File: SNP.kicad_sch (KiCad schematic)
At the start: 9 parts, among them J1 SNP, U75 IN74ALS32N (КР1533ЛЛ1)

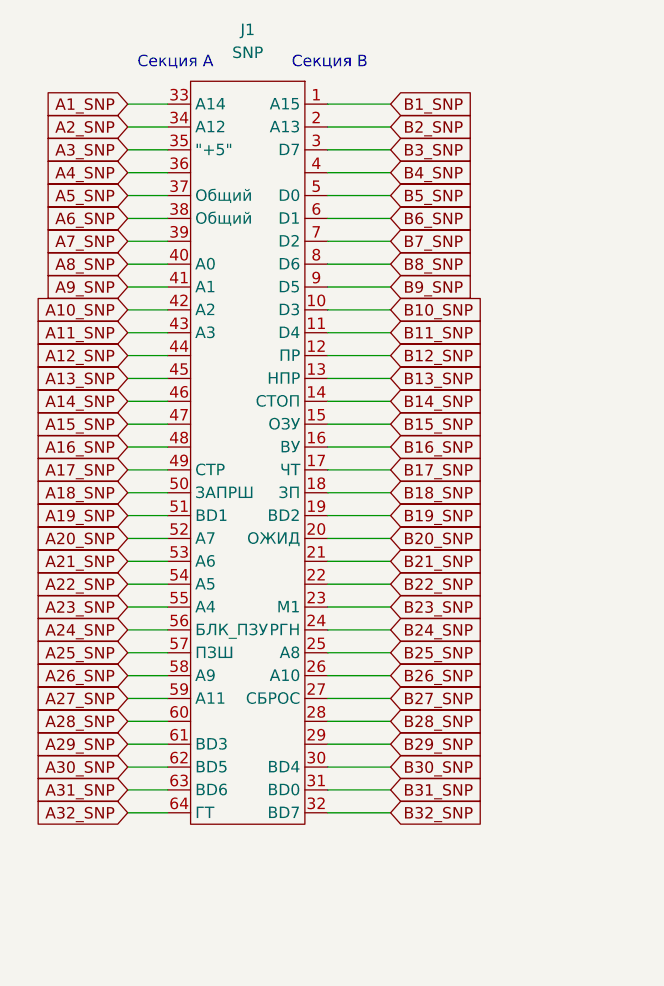
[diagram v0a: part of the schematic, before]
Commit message: March 22nd - 3rd edition
List 3 is complete
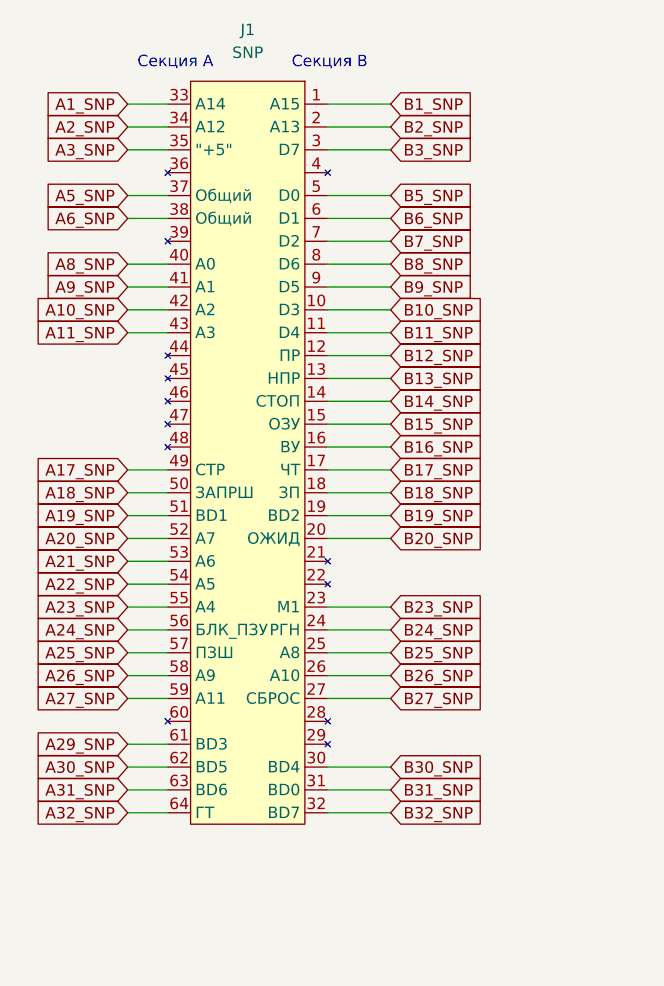
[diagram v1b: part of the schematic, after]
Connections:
- net GND: no longer J1.45
- net A12_SNP: no longer names the net of J1.44
- net A14_SNP: no longer names the net of J1.46
- net A15_SNP: no longer names the net of J1.47
- net A16_SNP: no longer names the net of J1.48
- net A28_SNP: no longer names the net of J1.60
- net A4_SNP: no longer names the net of J1.36
- net A7_SNP: no longer names the net of J1.39
- net B21_SNP: no longer names the net of J1.21
- net B22_SNP: no longer names the net of J1.22
- net B28_SNP: no longer names the net of J1.28
- net B29_SNP: no longer names the net of J1.29
- net B4_SNP: no longer names the net of J1.4
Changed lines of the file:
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@@
 (kicad_sch (version 20211123) (generator eeschema)
-  (paper "A3")
+  (paper "A4")
   (title_block
     (comment 2 "Евстафьев")
@@
     (stroke (width 0) (type default) (color 0 0 0 0))
   )
-  (wire (pts (xy 40.005 69.85) (xy 44.45 69.85))
-    (stroke (width 0) (type default) (color 0 0 0 0))
-  )
   (wire (pts (xy 173.99 46.355) (xy 173.99 50.165))
     (stroke (width 0) (type default) (color 0 0 0 0))
@@
     (stroke (width 0) (type default) (color 0 0 0 0))
   )
-  (wire (pts (xy 40.005 67.31) (xy 44.45 67.31))
-    (stroke (width 0) (type default) (color 0 0 0 0))
-  )
   (wire (pts (xy 138.43 46.355) (xy 138.43 70.485))
     (stroke (width 0) (type default) (color 0 0 0 0))
@@
     (stroke (width 0) (type default) (color 0 0 0 0))
   )
-  (wire (pts (xy 40.005 64.77) (xy 44.45 64.77))
-    (stroke (width 0) (type default) (color 0 0 0 0))
-  )
   (wire (pts (xy 128.27 46.355) (xy 128.27 60.325))
     (stroke (width 0) (type default) (color 0 0 0 0))
   )
-  (wire (pts (xy 69.215 85.09) (xy 62.23 85.09))
-    (stroke (width 0) (type default) (color 0 0 0 0))
-  )
   (wire (pts (xy 40.005 74.93) (xy 44.45 74.93))
     (stroke (width 0) (type default) (color 0 0 0 0))
@@
     (stroke (width 0) (type default) (color 0 0 0 0))
   )
-  (wire (pts (xy 69.215 102.87) (xy 62.23 102.87))
-    (stroke (width 0) (type default) (color 0 0 0 0))
-  )
   (wire (pts (xy 135.89 67.945) (xy 151.13 67.945))
     (stroke (width 0) (type default) (color 0 0 0 0))
@@
     (stroke (width 0) (type default) (color 0 0 0 0))
   )
-  (wire (pts (xy 40.005 62.23) (xy 44.45 62.23))
-    (stroke (width 0) (type default) (color 0 0 0 0))
-  )
   (wire (pts (xy 133.35 46.355) (xy 133.35 65.405))
     (stroke (width 0) (type default) (color 0 0 0 0))
@@
     (stroke (width 0) (type default) (color 0 0 0 0))
   )
-  (wire (pts (xy 40.005 49.53) (xy 44.45 49.53))
-    (stroke (width 0) (type default) (color 0 0 0 0))
-  )
   (wire (pts (xy 124.46 88.265) (xy 151.13 88.265))
     (stroke (width 0) (type default) (color 0 0 0 0))
@@
     (stroke (width 0) (type default) (color 0 0 0 0))
   )
-  (wire (pts (xy 69.215 105.41) (xy 62.23 105.41))
-    (stroke (width 0) (type default) (color 0 0 0 0))
-  )
   (wire (pts (xy 128.27 98.425) (xy 128.27 100.965))
     (stroke (width 0) (type default) (color 0 0 0 0))
@@
     (stroke (width 0) (type default) (color 0 0 0 0))
   )
-  (wire (pts (xy 40.005 72.39) (xy 44.45 72.39))
-    (stroke (width 0) (type default) (color 0 0 0 0))
-  )
   (wire (pts (xy 40.005 52.07) (xy 44.45 52.07))
     (stroke (width 0) (type default) (color 0 0 0 0))
   )
-  (wire (pts (xy 69.215 87.63) (xy 62.23 87.63))
-    (stroke (width 0) (type default) (color 0 0 0 0))
-  )
   (wire (pts (xy 124.46 78.105) (xy 146.05 78.105))
     (stroke (width 0) (type default) (color 0 0 0 0))
   )
-  (wire (pts (xy 69.215 41.91) (xy 62.23 41.91))
-    (stroke (width 0) (type default) (color 0 0 0 0))
-  )
   (wire (pts (xy 40.005 97.79) (xy 44.45 97.79))
     (stroke (width 0) (type default) (color 0 0 0 0))
@@
     (stroke (width 0) (type default) (color 0 0 0 0))
   )
-  (wire (pts (xy 40.005 102.87) (xy 44.45 102.87))
-    (stroke (width 0) (type default) (color 0 0 0 0))
-  )
   (wire (pts (xy 190.5 57.15) (xy 190.5 55.245))
     (stroke (width 0) (type default) (color 0 0 0 0))
@@
   )
   (wire (pts (xy 155.575 36.195) (xy 173.99 36.195))
-    (stroke (width 0) (type default) (color 0 0 0 0))
-  )
-  (wire (pts (xy 40.005 41.91) (xy 44.45 41.91))
     (stroke (width 0) (type default) (color 0 0 0 0))
   )
@@
     )
   )
-  (global_label "A7_SNP" (shape input) (at 40.005 49.53 180) (fields_autoplaced)
-    (effects (font (size 1.27 1.27)) (justify right))
-    (property "Intersheet References" "${INTERSHEET_REFS}" (id 0) (at 30.5162 49.4506 0)
-      (effects (font (size 1.27 1.27)) (justify right) hide)
-    )
-  )
-  (global_label "A16_SNP" (shape input) (at 40.005 72.39 180) (fields_autoplaced)
-    (effects (font (size 1.27 1.27)) (justify right))
-    (property "Intersheet References" "${INTERSHEET_REFS}" (id 0) (at 29.3067 72.3106 0)
-      (effects (font (size 1.27 1.27)) (justify right) hide)
-    )
-  )
   (global_label "A26_SNP" (shape input) (at 40.005 97.79 180) (fields_autoplaced)
     (effects (font (size 1.27 1.27)) (justify right))
@@
     )
   )
-  (global_label "B22_SNP" (shape input) (at 69.215 87.63 0) (fields_autoplaced)
-    (effects (font (size 1.27 1.27)) (justify left))
-    (property "Intersheet References" "${INTERSHEET_REFS}" (id 0) (at 80.0948 87.5506 0)
-      (effects (font (size 1.27 1.27)) (justify left) hide)
-    )
-  )
-  (global_label "B4_SNP" (shape input) (at 69.215 41.91 0) (fields_autoplaced)
-    (effects (font (size 1.27 1.27)) (justify left))
-    (property "Intersheet References" "${INTERSHEET_REFS}" (id 0) (at 78.8852 41.8306 0)
-      (effects (font (size 1.27 1.27)) (justify left) hide)
-    )
-  )
   (global_label "A18_SNP" (shape input) (at 40.005 77.47 180) (fields_autoplaced)
     (effects (font (size 1.27 1.27)) (justify right))
@@
     )
   )
-  (global_label "A12_SNP" (shape input) (at 40.005 62.23 180) (fields_autoplaced)
-    (effects (font (size 1.27 1.27)) (justify right))
-    (property "Intersheet References" "${INTERSHEET_REFS}" (id 0) (at 29.3067 62.1506 0)
-      (effects (font (size 1.27 1.27)) (justify right) hide)
-    )
-  )
   (global_label "ЗАПРШL" (shape input) (at 194.31 52.705 0) (fields_autoplaced)
     (effects (font (size 1.27 1.27)) (justify left))
@@
     )
   )
-  (global_label "A14_SNP" (shape input) (at 40.005 67.31 180) (fields_autoplaced)
-    (effects (font (size 1.27 1.27)) (justify right))
-    (property "Intersheet References" "${INTERSHEET_REFS}" (id 0) (at 29.3067 67.2306 0)
-      (effects (font (size 1.27 1.27)) (justify right) hide)
-    )
-  )
   (global_label "B9_SNP" (shape input) (at 69.215 54.61 0) (fields_autoplaced)
     (effects (font (size 1.27 1.27)) (justify left))
@@
     )
   )
-  (global_label "A28_SNP" (shape input) (at 40.005 102.87 180) (fields_autoplaced)
-    (effects (font (size 1.27 1.27)) (justify right))
-    (property "Intersheet References" "${INTERSHEET_REFS}" (id 0) (at 29.3067 102.7906 0)
-      (effects (font (size 1.27 1.27)) (justify right) hide)
-    )
-  )
   (global_label "A6_SNP" (shape input) (at 124.46 98.425 180) (fields_autoplaced)
     (effects (font (size 1.27 1.27)) (justify right))
@@
     )
   )
-  (global_label "B21_SNP" (shape input) (at 69.215 85.09 0) (fields_autoplaced)
-    (effects (font (size 1.27 1.27)) (justify left))
-    (property "Intersheet References" "${INTERSHEET_REFS}" (id 0) (at 80.0948 85.0106 0)
-      (effects (font (size 1.27 1.27)) (justify left) hide)
-    )
-  )
   (global_label "B9_SNP" (shape input) (at 124.46 73.025 180) (fields_autoplaced)
     (effects (font (size 1.27 1.27)) (justify right))
@@
     )
   )
-  (global_label "B29_SNP" (shape input) (at 69.215 105.41 0) (fields_autoplaced)
-    (effects (font (size 1.27 1.27)) (justify left))
-    (property "Intersheet References" "${INTERSHEET_REFS}" (id 0) (at 80.0948 105.3306 0)
-      (effects (font (size 1.27 1.27)) (justify left) hide)
-    )
-  )
   (global_label "B8_SNP" (shape input) (at 69.215 52.07 0) (fields_autoplaced)
     (effects (font (size 1.27 1.27)) (justify left))
@@
     )
   )
-  (global_label "B28_SNP" (shape input) (at 69.215 102.87 0) (fields_autoplaced)
-    (effects (font (size 1.27 1.27)) (justify left))
-    (property "Intersheet References" "${INTERSHEET_REFS}" (id 0) (at 80.0948 102.7906 0)
-      (effects (font (size 1.27 1.27)) (justify left) hide)
-    )
-  )
   (global_label "A29_SNP" (shape input) (at 40.005 105.41 180) (fields_autoplaced)
     (effects (font (size 1.27 1.27)) (justify right))
@@
     )
   )
-  (global_label "A15_SNP" (shape input) (at 40.005 69.85 180) (fields_autoplaced)
-    (effects (font (size 1.27 1.27)) (justify right))
-    (property "Intersheet References" "${INTERSHEET_REFS}" (id 0) (at 29.3067 69.7706 0)
-      (effects (font (size 1.27 1.27)) (justify right) hide)
-    )
-  )
   (global_label "A23_SNP" (shape input) (at 40.005 90.17 180) (fields_autoplaced)
     (effects (font (size 1.27 1.27)) (justify right))
@@
     )
   )
-  (global_label "A4_SNP" (shape input) (at 40.005 41.91 180) (fields_autoplaced)
-    (effects (font (size 1.27 1.27)) (justify right))
-    (property "Intersheet References" "${INTERSHEET_REFS}" (id 0) (at 30.5162 41.8306 0)
-      (effects (font (size 1.27 1.27)) (justify right) hide)
-    )
-  )
   (global_label "A30_SNP" (shape input) (at 40.005 107.95 180) (fields_autoplaced)
     (effects (font (size 1.27 1.27)) (justify right))
@@
     )
   )
-  (global_label "A13_SNP" (shape input) (at 40.005 64.77 180) (fields_autoplaced)
-    (effects (font (size 1.27 1.27)) (justify right))
-    (property "Intersheet References" "${INTERSHEET_REFS}" (id 0) (at 29.3067 64.6906 0)
-      (effects (font (size 1.27 1.27)) (justify right) hide)
-    )
-  )
